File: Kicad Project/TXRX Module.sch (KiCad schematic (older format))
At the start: 13 parts

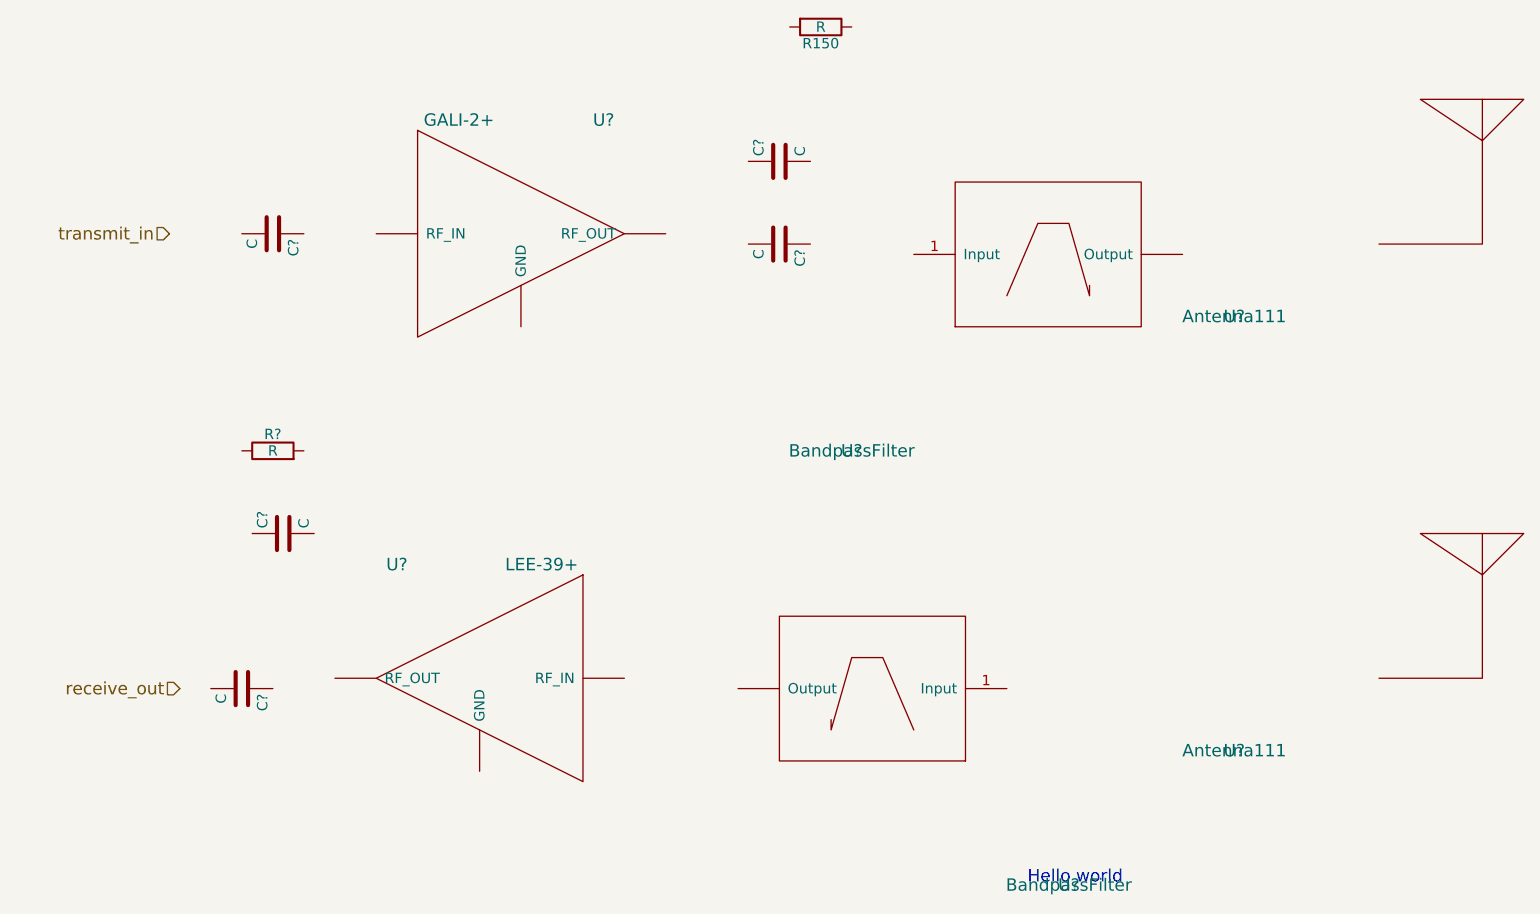
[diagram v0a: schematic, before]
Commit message: Connected stuffs and things
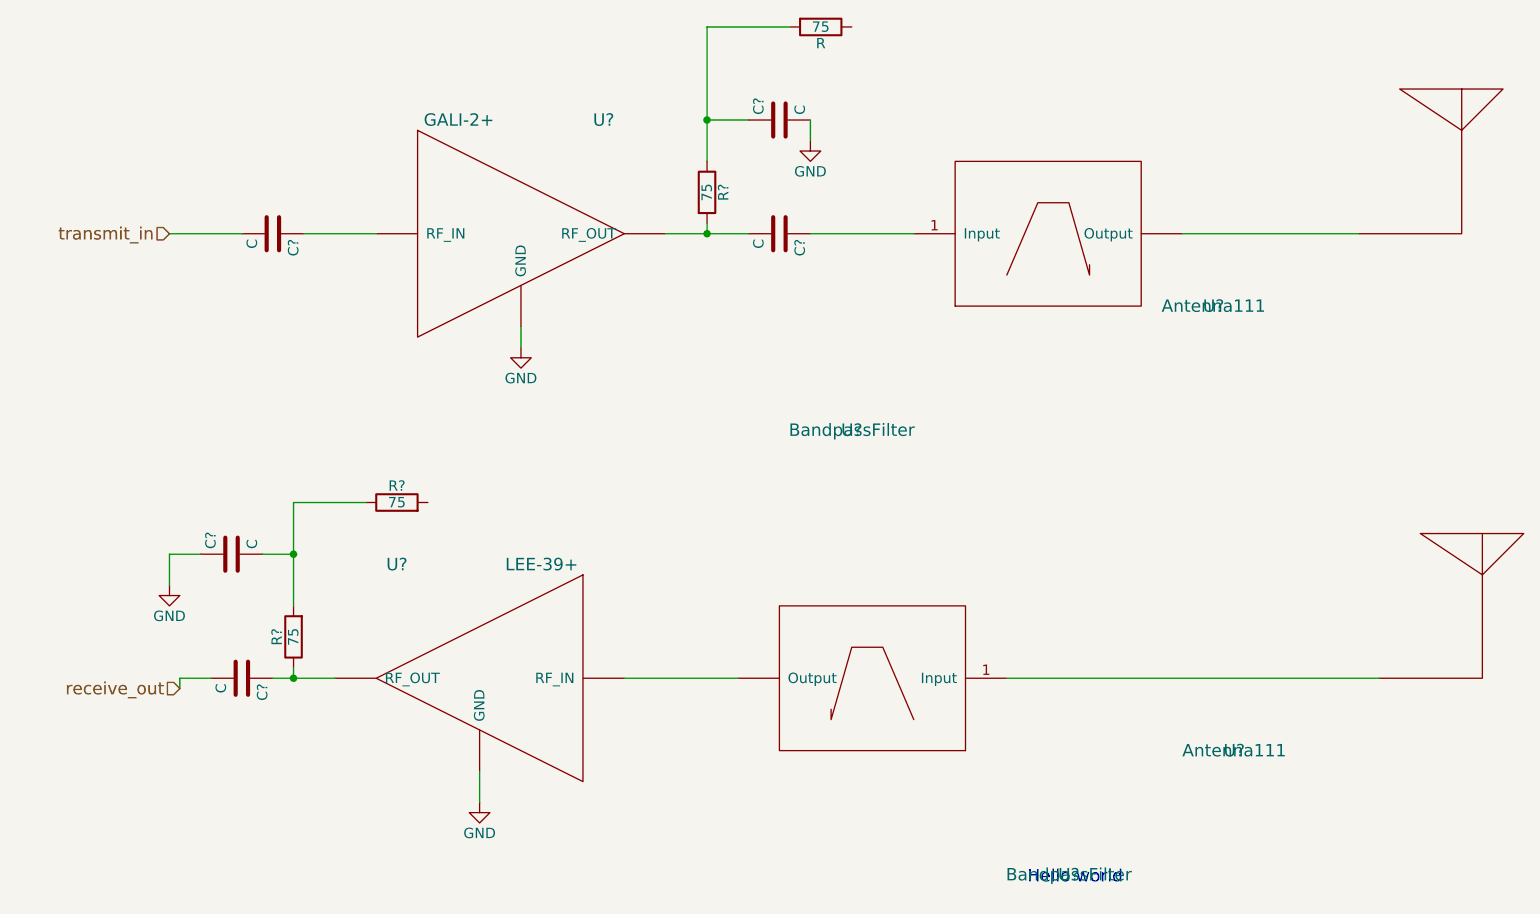
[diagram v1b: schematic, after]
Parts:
- removed R?: R, symbol R
- added R? (x3): 75, symbol R
- R: renamed from R150; value R -> 75
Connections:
- net labels added: GND
- wire segments 0 -> 23
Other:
- moved on the sheet: C?, U?
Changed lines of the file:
@@
 L C C?
 U 1 1 59FF6B4C
-P 5300 2300
-F 0 "C?" H 5325 2400 50  0000 L CNN
-F 1 "C" H 5325 2200 50  0000 L CNN
-F 2 "" H 5338 2150 50  0001 C CNN
-F 3 "" H 5300 2300 50  0001 C CNN
-	1    5300 2300
+P 5300 2100
+F 0 "C?" H 5325 2200 50  0000 L CNN
+F 1 "C" H 5325 2000 50  0000 L CNN
+F 2 "" H 5338 1950 50  0001 C CNN
+F 3 "" H 5300 2100 50  0001 C CNN
+	1    5300 2100
 	0    -1   -1   0
 $EndComp
@@
 $EndComp
 $Comp
-L R R150
+L R R
 U 1 1 59FF7053
 P 5500 1650
-F 0 "R150" V 5580 1650 50  0000 C CNN
-F 1 "R" V 5500 1650 50  0000 C CNN
+F 0 "R" V 5580 1650 50  0000 C CNN
+F 1 "75" V 5500 1650 50  0000 C CNN
 F 2 "" V 5430 1650 50  0001 C CNN
 F 3 "" H 5500 1650 50  0001 C CNN
@@
 L BandpassFilter U?
 U 1 1 59FF71CB
-P 5650 3700
-F 0 "U?" H 5650 3700 60  0000 C CNN
-F 1 "BandpassFilter" H 5650 3700 60  0000 C CNN
-F 2 "" H 5650 3700 60  0001 C CNN
-F 3 "" H 5650 3700 60  0001 C CNN
-	1    5650 3700
+P 5650 3600
+F 0 "U?" H 5650 3600 60  0000 C CNN
+F 1 "BandpassFilter" H 5650 3600 60  0000 C CNN
+F 2 "" H 5650 3600 60  0001 C CNN
+F 3 "" H 5650 3600 60  0001 C CNN
+	1    5650 3600
 	1    0    0    -1
 $EndComp
@@
 L BandpassFilter U?
 U 1 1 59FFC13A
-P 6700 5800
-F 0 "U?" H 6700 5800 60  0000 C CNN
-F 1 "BandpassFilter" H 6700 5800 60  0000 C CNN
-F 2 "" H 6700 5800 60  0001 C CNN
-F 3 "" H 6700 5800 60  0001 C CNN
-	1    6700 5800
+P 6700 5750
+F 0 "U?" H 6700 5750 60  0000 C CNN
+F 1 "BandpassFilter" H 6700 5750 60  0000 C CNN
+F 2 "" H 6700 5750 60  0001 C CNN
+F 3 "" H 6700 5750 60  0001 C CNN
+	1    6700 5750
 	-1   0    0    -1
 $EndComp
 $Comp
-L R R?
-U 1 1 59FFC214
-P 2850 3700
-F 0 "R?" V 2930 3700 50  0000 C CNN
-F 1 "R" V 2850 3700 50  0000 C CNN
-F 2 "" V 2780 3700 50  0001 C CNN
-F 3 "" H 2850 3700 50  0001 C CNN
-	1    2850 3700
+L C C?
+U 1 1 59FFC2C3
+P 2650 4200
+F 0 "C?" H 2675 4300 50  0000 L CNN
+F 1 "C" H 2675 4100 50  0000 L CNN
+F 2 "" H 2688 4050 50  0001 C CNN
+F 3 "" H 2650 4200 50  0001 C CNN
+	1    2650 4200
 	0    -1   -1   0
 $EndComp
 $Comp
 L C C?
-U 1 1 59FFC2C3
-P 2900 4100
-F 0 "C?" H 2925 4200 50  0000 L CNN
-F 1 "C" H 2925 4000 50  0000 L CNN
-F 2 "" H 2938 3950 50  0001 C CNN
-F 3 "" H 2900 4100 50  0001 C CNN
-	1    2900 4100
-	0    -1   -1   0
-$EndComp
-$Comp
-L C C?
 U 1 1 59FFC68E
-P 5300 2700
-F 0 "C?" H 5325 2800 50  0000 L CNN
-F 1 "C" H 5325 2600 50  0000 L CNN
-F 2 "" H 5338 2550 50  0001 C CNN
-F 3 "" H 5300 2700 50  0001 C CNN
-	1    5300 2700
+P 5300 2650
+F 0 "C?" H 5325 2750 50  0000 L CNN
+F 1 "C" H 5325 2550 50  0000 L CNN
+F 2 "" H 5338 2500 50  0001 C CNN
+F 3 "" H 5300 2650 50  0001 C CNN
+	1    5300 2650
 	0    1    1    0
 $EndComp
@@
 L C C?
 U 1 1 59FFC719
-P 2700 4850
-F 0 "C?" H 2725 4950 50  0000 L CNN
-F 1 "C" H 2725 4750 50  0000 L CNN
-F 2 "" H 2738 4700 50  0001 C CNN
-F 3 "" H 2700 4850 50  0001 C CNN
-	1    2700 4850
+P 2700 4800
+F 0 "C?" H 2725 4900 50  0000 L CNN
+F 1 "C" H 2725 4700 50  0000 L CNN
+F 2 "" H 2738 4650 50  0001 C CNN
+F 3 "" H 2700 4800 50  0001 C CNN
+	1    2700 4800
 	0    1    1    0
 $EndComp
@@
 L Antenna111 U?
 U 1 1 59FFCB61
-P 7500 3050
-F 0 "U?" H 7500 3050 60  0000 C CNN
-F 1 "Antenna111" H 7500 3050 60  0000 C CNN
-F 2 "" H 7500 3050 60  0001 C CNN
-F 3 "" H 7500 3050 60  0001 C CNN
-	1    7500 3050
+P 7400 3000
+F 0 "U?" H 7400 3000 60  0000 C CNN
+F 1 "Antenna111" H 7400 3000 60  0000 C CNN
+F 2 "" H 7400 3000 60  0001 C CNN
+F 3 "" H 7400 3000 60  0001 C CNN
+	1    7400 3000
 	1    0    0    -1
 $EndComp
@@
 	1    0    0    -1
 $EndComp
+$Comp
+L R R?
+U 1 1 59FFDD37
+P 4950 2450
+F 0 "R?" V 5030 2450 50  0000 C CNN
+F 1 "75" V 4950 2450 50  0000 C CNN
+F 2 "" V 4880 2450 50  0001 C CNN
+F 3 "" H 4950 2450 50  0001 C CNN
+	1    4950 2450
+	1    0    0    -1
+$EndComp
+Wire Wire Line
+	2350 2650 2700 2650
+Wire Wire Line
+	3000 2650 3350 2650
+Wire Wire Line
+	4750 2650 5150 2650
+Wire Wire Line
+	5450 2650 5950 2650
+Wire Wire Line
+	4950 2600 4950 2650
+Connection ~ 4950 2650
+Wire Wire Line
+	4950 1650 4950 2300
+Wire Wire Line
+	4950 2100 5150 2100
+Wire Wire Line
+	4950 1650 5350 1650
+Connection ~ 4950 2100
+Wire Wire Line
+	8100 2650 7250 2650
+$Comp
+L R R?
+U 1 1 59FFE442
+P 3450 3950
+F 0 "R?" V 3530 3950 50  0000 C CNN
+F 1 "75" V 3450 3950 50  0000 C CNN
+F 2 "" V 3380 3950 50  0001 C CNN
+F 3 "" H 3450 3950 50  0001 C CNN
+	1    3450 3950
+	0    -1   -1   0
+$EndComp
+$Comp
+L R R?
+U 1 1 59FFE542
+P 2950 4600
+F 0 "R?" V 3030 4600 50  0000 C CNN
+F 1 "75" V 2950 4600 50  0000 C CNN
+F 2 "" V 2880 4600 50  0001 C CNN
+F 3 "" H 2950 4600 50  0001 C CNN
+	1    2950 4600
+	-1   0    0    1
+$EndComp
+$Comp
+L GND #PWR?
+U 1 1 59FFE5A2
+P 2350 4350
+F 0 "#PWR?" H 2350 4100 50  0001 C CNN
+F 1 "GND" H 2350 4200 50  0000 C CNN
+F 2 "" H 2350 4350 50  0001 C CNN
+F 3 "" H 2350 4350 50  0001 C CNN
+	1    2350 4350
+	1    0    0    -1
+$EndComp
+$Comp
+L GND #PWR?
+U 1 1 59FFE5D4
+P 3850 5400
+F 0 "#PWR?" H 3850 5150 50  0001 C CNN
+F 1 "GND" H 3850 5250 50  0000 C CNN
+F 2 "" H 3850 5400 50  0001 C CNN
+F 3 "" H 3850 5400 50  0001 C CNN
+	1    3850 5400
+	1    0    0    -1
+$EndComp
+$Comp
+L GND #PWR?
+U 1 1 59FFE606
+P 4050 3200
+F 0 "#PWR?" H 4050 2950 50  0001 C CNN
+F 1 "GND" H 4050 3050 50  0000 C CNN
+F 2 "" H 4050 3200 50  0001 C CNN
+F 3 "" H 4050 3200 50  0001 C CNN
+	1    4050 3200
+	1    0    0    -1
+$EndComp
+$Comp
+L GND #PWR?
+U 1 1 59FFE638
+P 5450 2200
+F 0 "#PWR?" H 5450 1950 50  0001 C CNN
+F 1 "GND" H 5450 2050 50  0000 C CNN
+F 2 "" H 5450 2200 50  0001 C CNN
+F 3 "" H 5450 2200 50  0001 C CNN
+	1    5450 2200
+	1    0    0    -1
+$EndComp
+Wire Wire Line
+	8200 4800 6400 4800
+Wire Wire Line
+	5100 4800 4550 4800
+Wire Wire Line
+	3150 4800 2850 4800
+Wire Wire Line
+	2950 4750 2950 4800
+Connection ~ 2950 4800
+Wire Wire Line
+	2950 4450 2950 3950
+Wire Wire Line
+	2950 3950 3300 3950
+Wire Wire Line
+	2800 4200 2950 4200
+Connection ~ 2950 4200
+Wire Wire Line
+	2500 4200 2350 4200
+Wire Wire Line
+	2350 4200 2350 4350
+Wire Wire Line
+	3850 5250 3850 5400
+Wire Wire Line
+	5450 2100 5450 2200
+Wire Wire Line
+	4050 3100 4050 3200
+Wire Wire Line
+	2550 4800 2400 4800
+Wire Wire Line
+	2400 4800 2400 4850
 $EndSCHEMATC
